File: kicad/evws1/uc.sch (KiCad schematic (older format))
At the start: 64 parts, among them J13 atmega-isp-6, J14 header, M5 rpi-ev-plc-adapter-v1.0, Q3 AO3400, SW3 SW_Push, SW4 dip-switch-4x2pos-smd-1.27mm, SW5 SS-12D00G3, U1 atmega324p-20au, U4 PCF8591, U7 DS1307ZN, U8 24LC512, U9 PCF8574, Y1 20MHz, Y4 32768kHz

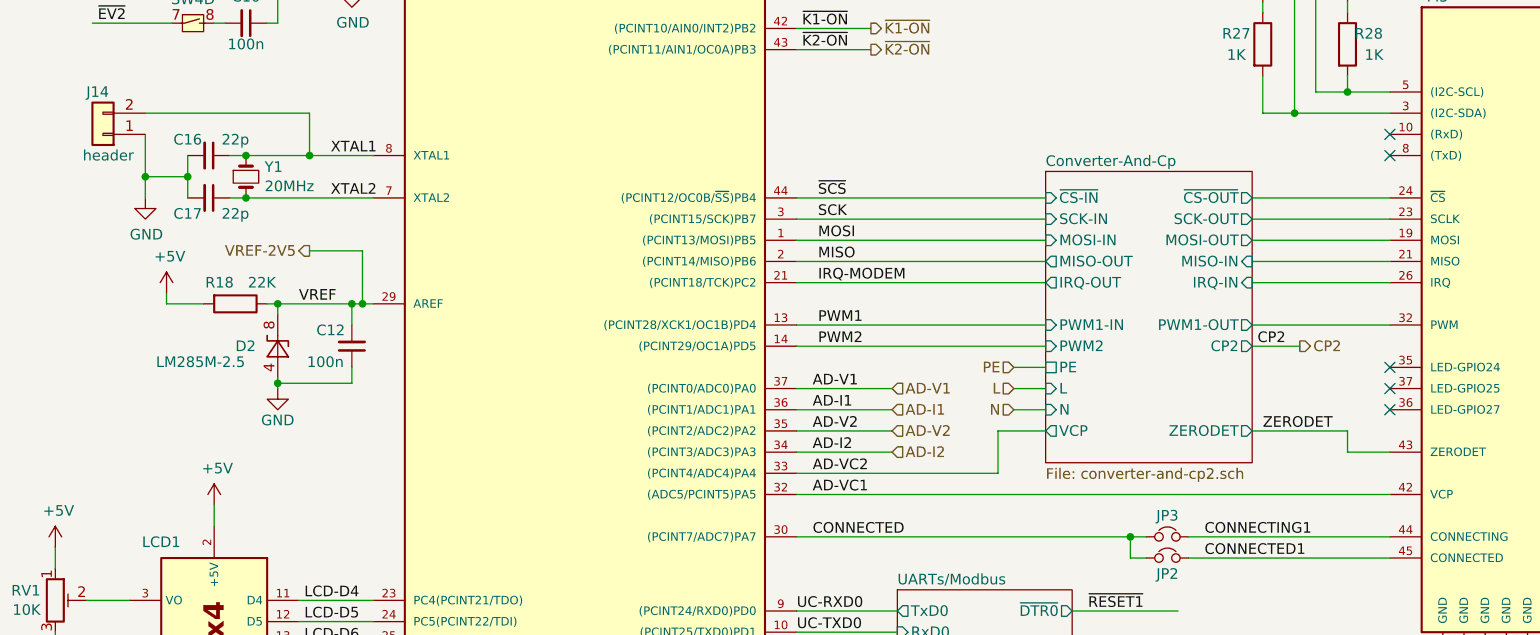
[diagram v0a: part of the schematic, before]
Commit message: ...
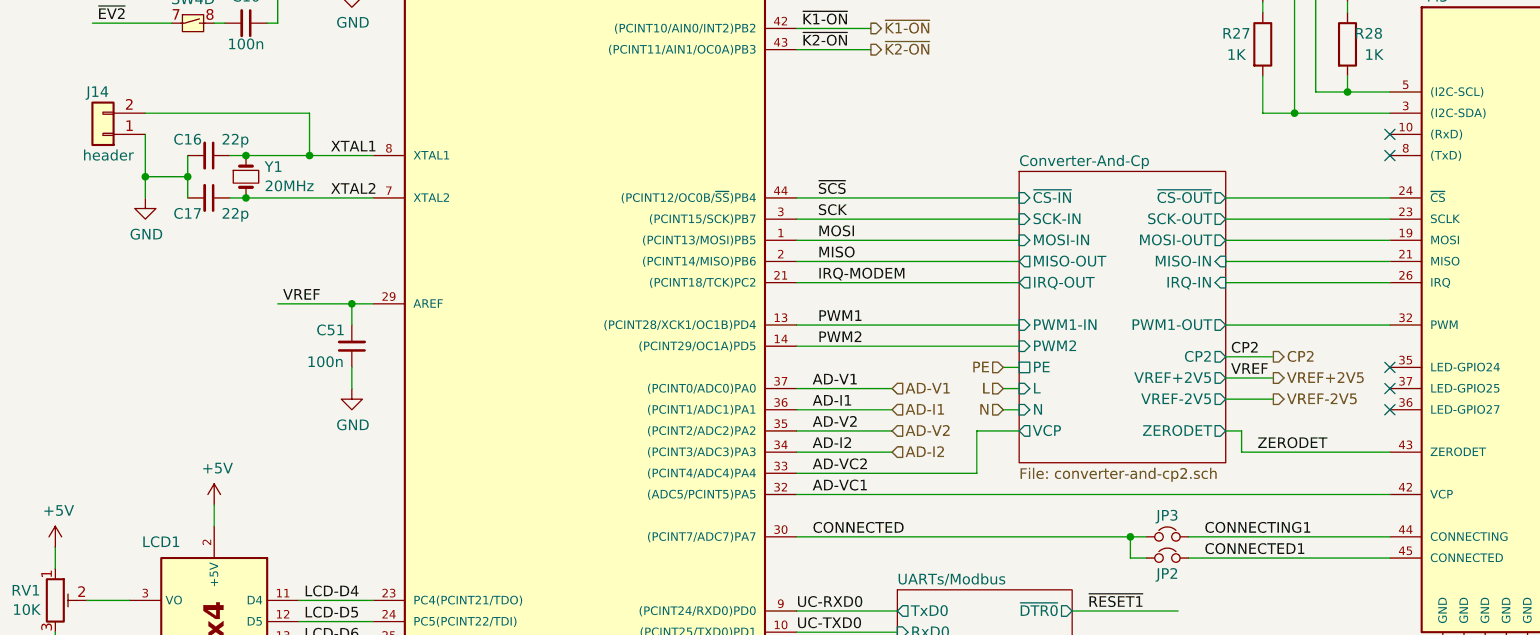
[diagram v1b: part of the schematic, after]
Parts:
- removed D2: LM285M-2.5, Project:SOIC-8_3.9x4.9mm_Pitch1.27mm_Handsolded, symbol _project:LM285M-2.5
- removed R18: 22K, Project:r-0805-hand-soldering, symbol Device:R
- renumbered C12 to C51
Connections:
- net labels added: VREF+2V5
- wire segments 356 -> 348
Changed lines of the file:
@@
 Text Label 3350 1550 0    50   ~ 0
 AVCC
-$Comp
-L _project:LM285M-2.5 D2
-U 1 1 5E164F25
-P 1850 4350
-F 0 "D2" V 1850 4550 50  0000 R CNN
-F 1 "LM285M-2.5" V 1775 4925 50  0000 R CNN
-F 2 "Project:SOIC-8_3.9x4.9mm_Pitch1.27mm_Handsolded" H 1850 4150 50  0001 C CIN
-F 3 "" H 1850 4350 50  0001 C CIN
-	1    1850 4350
-	0    -1   -1   0
-$EndComp
-$Comp
-L power:GND #PWR?
-U 1 1 5E165204
-P 1850 4550
-AR Path="/5E165204" Ref="#PWR?"  Part="1"
-AR Path="/5E0A3961/5E165204" Ref="#PWR0139"  Part="1"
-F 0 "#PWR0139" H 1850 4300 50  0001 C CNN
-F 1 "GND" H 1850 4400 50  0000 C CNN
-F 2 "" H 1850 4550 50  0001 C CNN
-F 3 "" H 1850 4550 50  0001 C CNN
-	1    1850 4550
-	1    0    0    -1
-$EndComp
-$Comp
-L Device:R R18
-U 1 1 5E1652F1
-P 1650 4150
-F 0 "R18" V 1550 4075 50  0000 C CNN
-F 1 "22K" V 1550 4275 50  0000 C CNN
-F 2 "Project:r-0805-hand-soldering" V 1580 4150 50  0001 C CNN
-F 3 "~" H 1650 4150 50  0001 C CNN
-	1    1650 4150
-	0    1    1    0
-$EndComp
-Wire Wire Line
-	1500 4150 1325 4150
-Wire Wire Line
-	1325 4150 1325 4100
-Wire Wire Line
-	1800 4150 1850 4150
-Wire Wire Line
-	1850 4150 1850 4200
-Wire Wire Line
-	1850 4500 1850 4525
-Connection ~ 1850 4150
-Text Label 1950 4150 0    50   ~ 0
-VREF
 Text Label 2100 3650 0    50   ~ 0
 XTAL2
 $Comp
-L Device:C_Small C12
+L Device:C_Small C51
 U 1 1 5E17379F
 P 2200 4350
-F 0 "C12" H 2300 4275 50  0000 C CNN
+F 0 "C51" H 2300 4275 50  0000 C CNN
 F 1 "100n" H 2325 4425 50  0000 C CNN
 F 2 "Project:c-1206-hand-soldering" H 2200 4350 50  0001 C CNN
@@
 $EndComp
 Wire Wire Line
-	2200 4450 2200 4525
-Wire Wire Line
-	2200 4525 1850 4525
-Connection ~ 1850 4525
-Wire Wire Line
-	1850 4525 1850 4550
+	2200 4450 2200 4550
 Wire Wire Line
 	2200 4250 2200 4150
-Connection ~ 2200 4150
-Wire Wire Line
-	2200 4150 2250 4150
 $Comp
 L power:GND #PWR?
@@
 F 3 "" H 1850 1000 50  0001 C CNN
 	1    1850 1000
-	1    0    0    -1
-$EndComp
-$Comp
-L power:+5V #PWR?
-U 1 1 5E28AA1E
-P 1325 4100
-AR Path="/5E28AA1E" Ref="#PWR?"  Part="1"
-AR Path="/5E0A3961/5E28AA1E" Ref="#PWR0145"  Part="1"
-F 0 "#PWR0145" H 1325 3950 50  0001 C CNN
-F 1 "+5V" H 1340 4273 50  0000 C CNN
-F 2 "" H 1325 4100 50  0001 C CNN
-F 3 "" H 1325 4100 50  0001 C CNN
-	1    1325 4100
 	1    0    0    -1
 $EndComp
@@
 Text Label 8475 1200 0    50   ~ 0
 AOUT
-Text HLabel 2000 3900 0    50   Output ~ 0
-VREF-2V5
+Text HLabel 6550 4500 2    50   Output ~ 0
+VREF+2V5
 Wire Wire Line
 	7850 2250 9800 2250
@@
 Wire Wire Line
 	7100 5250 6150 5250
-Text HLabel 6675 4350 2    50   Output ~ 0
+Text HLabel 6550 4400 2    50   Output ~ 0
 CP2
 Wire Wire Line
-	6675 4350 6450 4350
+	6550 4400 6325 4400
 Text HLabel 9550 4750 2    50   Output ~ 0
 CP1
-Text Label 6475 4350 0    50   ~ 0
+Text Label 6350 4400 0    50   ~ 0
 CP2
 Text Label 4400 4350 0    50   ~ 0
@@
 Wire Wire Line
 	6000 7050 6000 7000
-Text Label 6500 4750 0    50   ~ 0
+Text Label 6475 4850 0    50   ~ 0
 ZERODET
 Text Label 6225 5250 0    50   ~ 0
@@
 Text Label 6225 5350 0    50   ~ 0
 CONNECTED1
-Wire Wire Line
-	1850 4150 2200 4150
 Text Label 4375 5250 0    50   ~ 0
 CONNECTED
@@
 Text Label 4375 4950 0    50   ~ 0
 AD-VC2
-Text HLabel 5325 4450 0    50   Input ~ 0
+Text HLabel 5275 4450 0    50   Input ~ 0
 PE
 NoConn ~ 8650 5850
@@
 	5600 6200 5850 6200
 $Sheet
-S 5475 3525 975  1375
+S 5350 3525 975  1375
 U 5E29AFD8
 F0 "Converter-And-Cp" 50
 F1 "converter-and-cp2.sch" 50
-F2 "PE" U L 5475 4450 50
-F3 "VCP" O L 5475 4750 50
-F4 "ZERODET" O R 6450 4750 50
-F5 "L" I L 5475 4550 50
-F6 "N" I L 5475 4650 50
-F7 "PWM2" I L 5475 4350 50
-F8 "CP2" O R 6450 4350 50
-F9 "~CS-IN" I L 5475 3650 50
-F10 "SCK-IN" I L 5475 3750 50
-F11 "MOSI-IN" I L 5475 3850 50
-F12 "MISO-IN" I R 6450 3950 50
-F13 "IRQ-IN" I R 6450 4050 50
-F14 "~CS-OUT" O R 6450 3650 50
-F15 "SCK-OUT" O R 6450 3750 50
-F16 "MOSI-OUT" O R 6450 3850 50
-F17 "MISO-OUT" O L 5475 3950 50
-F18 "IRQ-OUT" O L 5475 4050 50
-F19 "PWM1-IN" I L 5475 4250 50
-F20 "PWM1-OUT" O R 6450 4250 50
+F2 "PE" U L 5350 4450 50
+F3 "VCP" O L 5350 4750 50
+F4 "ZERODET" O R 6325 4750 50
+F5 "L" I L 5350 4550 50
+F6 "N" I L 5350 4650 50
+F7 "PWM2" I L 5350 4350 50
+F8 "CP2" O R 6325 4400 50
+F9 "~CS-IN" I L 5350 3650 50
+F10 "SCK-IN" I L 5350 3750 50
+F11 "MOSI-IN" I L 5350 3850 50
+F12 "MISO-IN" I R 6325 3950 50
+F13 "IRQ-IN" I R 6325 4050 50
+F14 "~CS-OUT" O R 6325 3650 50
+F15 "SCK-OUT" O R 6325 3750 50
+F16 "MOSI-OUT" O R 6325 3850 50
+F17 "MISO-OUT" O L 5350 3950 50
+F18 "IRQ-OUT" O L 5350 4050 50
+F19 "PWM1-IN" I L 5350 4250 50
+F20 "PWM1-OUT" O R 6325 4250 50
+F21 "VREF+2V5" O R 6325 4500 50
+F22 "VREF-2V5" O R 6325 4600 50
 $EndSheet
 Wire Wire Line
-	4300 4250 5475 4250
-Wire Wire Line
-	4300 4350 5475 4350
-Wire Wire Line
-	6450 4250 7100 4250
-Wire Wire Line
-	5475 4450 5325 4450
+	4300 4250 5350 4250
+Wire Wire Line
+	4300 4350 5350 4350
+Wire Wire Line
+	6325 4250 7100 4250
+Wire Wire Line
+	5350 4450 5275 4450
 Wire Wire Line
 	9750 3700 9750 3550
@@
 	9750 4050 9750 4000
 Connection ~ 9550 3350
-Text HLabel 5325 4550 0    50   Input ~ 0
+Text HLabel 5275 4550 0    50   Input ~ 0
 L
-Text HLabel 5325 4650 0    50   Input ~ 0
+Text HLabel 5275 4650 0    50   Input ~ 0
 N
 Wire Wire Line
-	5325 4550 5475 4550
-Wire Wire Line
-	5325 4650 5475 4650
-Wire Wire Line
-	5475 4750 5250 4750
-Wire Wire Line
-	5250 4750 5250 4950
-Wire Wire Line
-	4300 4950 5250 4950
-Wire Wire Line
-	4300 3650 5475 3650
-Wire Wire Line
-	4300 3750 5475 3750
-Wire Wire Line
-	4300 3850 5475 3850
-Wire Wire Line
-	4300 3950 5475 3950
-Wire Wire Line
-	4300 4050 5475 4050
-Wire Wire Line
-	6450 4750 6900 4750
+	5275 4550 5350 4550
+Wire Wire Line
+	5275 4650 5350 4650
+Wire Wire Line
+	5350 4750 5150 4750
+Wire Wire Line
+	5150 4750 5150 4950
+Wire Wire Line
+	4300 4950 5150 4950
+Wire Wire Line
+	4300 3650 5350 3650
+Wire Wire Line
+	4300 3750 5350 3750
+Wire Wire Line
+	4300 3850 5350 3850
+Wire Wire Line
+	4300 3950 5350 3950
+Wire Wire Line
+	4300 4050 5350 4050
+Wire Wire Line
+	6325 4750 6400 4750
 Connection ~ 6650 2350
 Wire Wire Line
@@
 	6750 3150 6900 3150
 Wire Wire Line
-	6900 4750 6900 4850
-Wire Wire Line
-	6900 4850 7100 4850
-Wire Wire Line
-	6450 4050 7100 4050
-Wire Wire Line
-	6450 3950 7100 3950
-Wire Wire Line
-	6450 3850 7100 3850
-Wire Wire Line
-	6450 3750 7100 3750
-Wire Wire Line
-	6450 3650 7100 3650
-Wire Wire Line
-	2250 4150 2250 3900
-Wire Wire Line
-	2250 3900 2000 3900
-Connection ~ 2250 4150
-Wire Wire Line
-	2250 4150 2300 4150
+	6400 4750 6400 4850
+Wire Wire Line
+	6400 4850 7100 4850
+Wire Wire Line
+	6325 4050 7100 4050
+Wire Wire Line
+	6325 3950 7100 3950
+Wire Wire Line
+	6325 3850 7100 3850
+Wire Wire Line
+	6325 3750 7100 3750
+Wire Wire Line
+	6325 3650 7100 3650
 Text Label 4300 5600 0    50   ~ 0
 UC-RXD0
@@
 Text Label 4300 6250 0    50   ~ 0
 UC-TXD1
+Wire Wire Line
+	2200 4150 2300 4150
+Text HLabel 6550 4600 2    50   Output ~ 0
+VREF-2V5
+Wire Wire Line
+	6325 4500 6550 4500
+Wire Wire Line
+	6325 4600 6550 4600
+Text Label 6350 4500 0    50   ~ 0
+VREF
+Wire Wire Line
+	2200 4150 1850 4150
+Connection ~ 2200 4150
+Text Label 1875 4150 0    50   ~ 0
+VREF
+$Comp
+L power:GND #PWR?
+U 1 1 5E66E279
+P 2200 4550
+AR Path="/5E66E279" Ref="#PWR?"  Part="1"
+AR Path="/5E0A3961/5E66E279" Ref="#PWR0240"  Part="1"
+F 0 "#PWR0240" H 2200 4300 50  0001 C CNN
+F 1 "GND" H 2205 4377 50  0000 C CNN
+F 2 "" H 2200 4550 50  0001 C CNN
+F 3 "" H 2200 4550 50  0001 C CNN
+	1    2200 4550
+	1    0    0    -1
+$EndComp
 $EndSCHEMATC
